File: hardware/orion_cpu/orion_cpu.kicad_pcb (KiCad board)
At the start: 2 copper layers, 99.7 x 99.7 mm, 74 parts, among them J1 C96ABC, J2 JTAG, SW1 CONFIG, SW2 ROM1, SW3 RESET

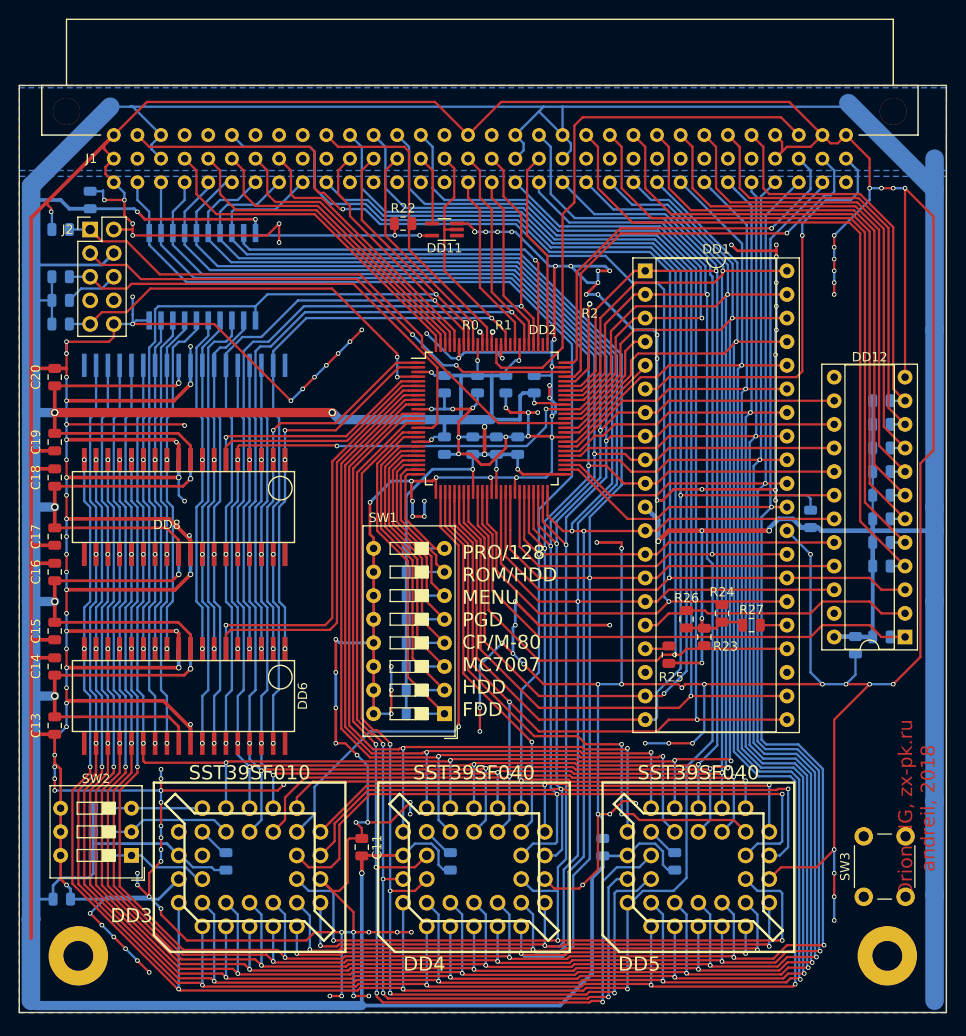
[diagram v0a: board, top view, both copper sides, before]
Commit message: RC версия процессорного модуля
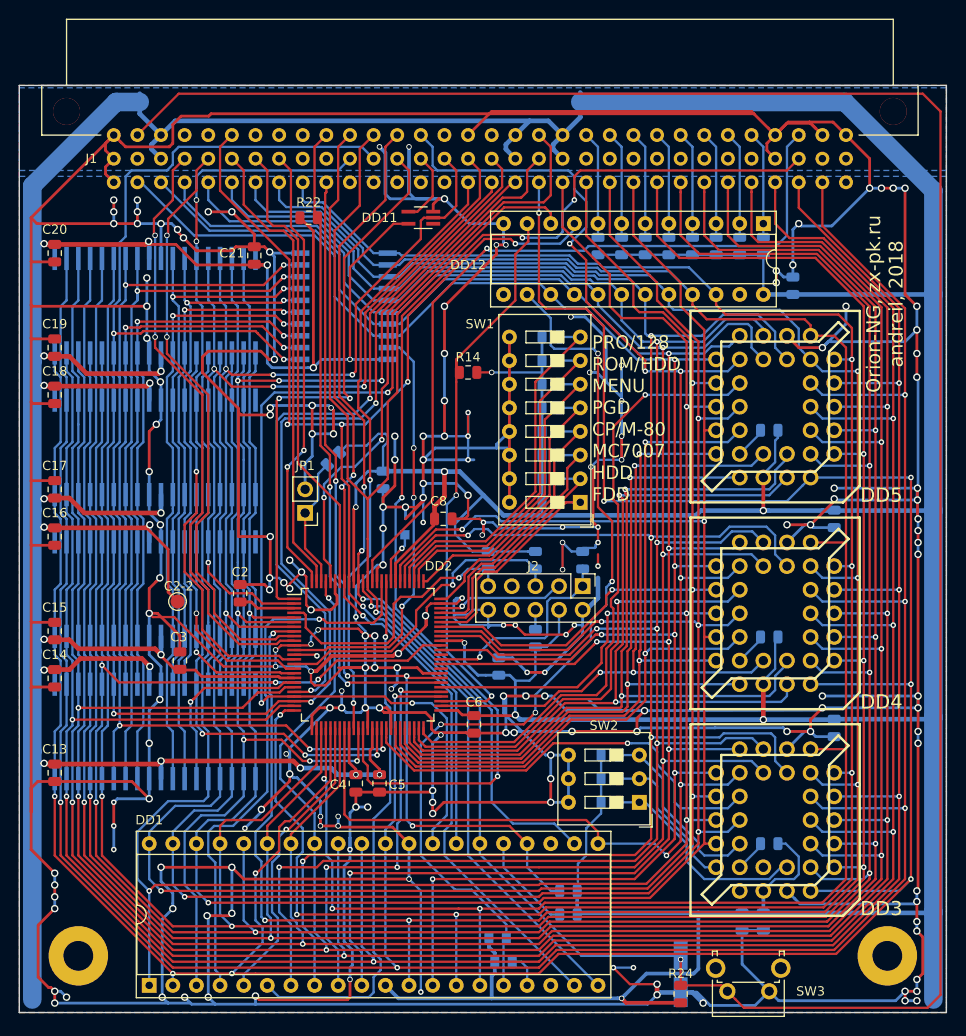
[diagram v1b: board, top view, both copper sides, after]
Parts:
- added C2-2: TestPoint_Pad_D1.5mm, TestPoint:TestPoint_Pad_D1.5mm, F.Cu at (86.9, 95.2)
- added C23: CP, Capacitors_Tantalum_SMD:CP_Tantalum_Case-A_EIA-3216-18_Hand, B.Cu at (141.0, 135.3)
- added JP1: R16B, Pin_Headers:Pin_Header_Straight_1x02_Pitch2.54mm, F.Cu at (100.6, 85.7)
- added R34: 1K, Resistor_SMD:R_0805_2012Metric, B.Cu at (103.6, 79.9)
- added REF**: TestPoint_Pad_1.0x1.0mm, TestPoint:TestPoint_Pad_1.0x1.0mm, B.Cu at (111.3, 88.1)
- C11, DD6, DD8, R23, R25, R26, R27: moved to B.Cu
- C2, C21, C3, C4, C5, C6, C8, R14: moved to F.Cu
- SW3: footprint Buttons_Switches_ThroughHole:SW_PUSH_6mm -> Button_Switch_THT:SW_Tactile_SPST_Angled_PTS645Vx83-2LFS
- moved DD1 93.5 mm to (83.8, 136.5), turned to 90 degrees
- moved C10 75.5 mm to (149.9, 129.7), turned to 90 degrees
- moved R32 66.4 mm to (130.4, 90.8), turned to 270 degrees
- moved J2 65.4 mm to (130.4, 93.6), turned to 270 degrees
- moved R29 62.7 mm to (125.3, 99.2), turned to 90 degrees
- moved R30 59.5 mm to (125.3, 90.8), turned to 270 degrees
- moved R12 58.5 mm to (150.5, 121.3), turned to 180 degrees
- moved DD3 56.7 mm to (151.1, 118.7), turned to 0 degrees
- moved R10 54.9 mm to (133.3, 114.3)
- moved R11 54.9 mm to (133.3, 111.8)
- moved R9 54.9 mm to (133.3, 116.8)
- moved SW2 54.9 mm to (136.5, 116.8)
- moved R14 52.8 mm to (118.1, 70.6), turned to 180 degrees
- moved R31 52.5 mm to (120.3, 90.8), turned to 270 degrees
- moved C11 52.4 mm to (157.5, 108.8), turned to 90 degrees
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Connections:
- net Net-(DD3-Pad31) renamed /PGM1
- net Net-(DD4-Pad31) renamed /PGM2
- net Net-(DD5-Pad31) renamed /PGM3
- DD10 pad 11: /D7 -> /D0
- DD10 pad 12: /D6 -> /D1
- DD10 pad 13: /D5 -> /D2
- DD10 pad 14: /D4 -> /D3
- DD10 pad 15: /D3 -> /D4
- DD10 pad 16: /D2 -> /D5
- DD10 pad 17: /D1 -> /D6
- DD10 pad 18: /D0 -> /D7
- DD10 pad 2: /MD7 -> /MD3
- DD10 pad 3: /MD0 -> /MD2
- DD10 pad 4: /MD6 -> /MD1
- DD10 pad 5: /MD1 -> /MD0
- DD10 pad 6: /MD2 -> /MD7
- DD10 pad 7: /MD5 -> /MD6
- DD10 pad 8: /MD3 -> /MD5
- DD12 pad 1: /~IRQ0 -> /~IRQS
- DD12 pad 10: /~IRQ7 -> /~IORQ
- DD12 pad 11: /~IRQS -> /~IRQ0
- DD12 pad 14: /D4 -> /~INT
- DD12 pad 15: /D3 -> /D7
- DD12 pad 16: /D5 -> /D6
- DD12 pad 17: /D6 -> /D5
- DD12 pad 18: /~IORQ -> /D4
- DD12 pad 19: /D2 -> /D3
- DD12 pad 2: /~INT -> /~IRQ7
- DD12 pad 20: /D7 -> /D2
- DD12 pad 21: /D0 -> /D1
- DD12 pad 22: /D1 -> /D0
- DD12 pad 3: /~M1 -> /~IRQ6
- DD12 pad 4: /~IRQ1 -> /~IRQ5
- DD12 pad 5: /~IRQ2 -> /~IRQ4
- DD12 pad 7: /~IRQ4 -> /~IRQ2
- DD12 pad 8: /~IRQ5 -> /~IRQ1
- DD12 pad 9: /~IRQ6 -> /~M1
- DD2 pad 1: /MA17 -> /~VCE
- DD2 pad 10: /R2A14 -> /~VO0
- DD2 pad 100: /~VO0 -> /pFA
- DD2 pad 12: /R2A17 -> /~OE0
- DD2 pad 13: /R2A18 -> /~OE1
- DD2 pad 14: /R2A16 -> /~CE0
- DD2 pad 16: /R2A15 -> /~CE1
- DD2 pad 17: /CFG0 -> /~CE2
- DD2 pad 19: /CFG1 -> /~CE3
- DD2 pad 2: /MA18 -> /MA15
- DD2 pad 20: /CFG2 -> /A2
- DD2 pad 21: /CFG3 -> /A14
- DD2 pad 22: /CFG4 -> /~RFSH
- DD2 pad 23: /CFG5 -> /MA14
- DD2 pad 24: /CFG6 -> /A1
- DD2 pad 25: /CFG7 -> /D0
- DD2 pad 27: /~R1 -> /A7
- DD2 pad 28: /~R2 -> /A5
- DD2 pad 29: /~R3 -> /D1
- DD2 pad 30: /~RD -> /A12
- DD2 pad 31: /~IORQ -> /ZA15
- DD2 pad 32: /~WR -> /A4
- DD2 pad 33: /~MREQ -> /~RD
- DD2 pad 35: /~WAIT -> /A15
- DD2 pad 36: /~IRQ0 -> /A13
- DD2 pad 37: /~RES -> /INT50
- DD2 pad 40: /D1 -> /~MRD
- DD2 pad 41: /~M1 -> /~MWR
- DD2 pad 42: /D0 -> /~R1
- DD2 pad 44: /~RFSH -> /R2A13
- DD2 pad 45: /D7 -> /R2A14
- DD2 pad 46: /D6 -> /R2A17
- DD2 pad 47: /D5 -> /R2A15
- DD2 pad 48: /D4 -> /R2A16
- DD2 pad 49: /D3 -> /~R2
- DD2 pad 5: /~CE3 -> /MA18
- DD2 pad 50: /D2 -> /~R3
- DD2 pad 52: /A0 -> /R2A18
- DD2 pad 53: /A1 -> /~IRQ0
- DD2 pad 54: /A2 -> /A0
- DD2 pad 55: /A3 -> /D5
- DD2 pad 56: /A4 -> /A11
- DD2 pad 57: /A5 -> /~BLIO
- DD2 pad 58: /A6 -> /~WAIT
- DD2 pad 6: /~CE2 -> /MA17
- DD2 pad 60: /ZA15 -> /CSL
- DD2 pad 61: /A7 -> /D6
- DD2 pad 63: /ZA14 -> /pFB
- DD2 pad 64: /A8 -> /D7
- DD2 pad 65: /A13 -> /A6
- DD2 pad 67: /A9 -> /D4
- DD2 pad 68: /A12 -> /A9
- DD2 pad 7: /~CE1 -> /MA16
- DD2 pad 70: /A11 -> /CFG0
- DD2 pad 71: /r2 -> /CFG1
- DD2 pad 72: /~TRB -> /CFG2
- DD2 pad 75: /INT50 -> /CFG3
- DD2 pad 76: /SND -> /CFG4
- DD2 pad 77: Net-(DD2-Pad77) -> /CFG5
- DD2 pad 78: /~OE0 -> /CFG6
- DD2 pad 79: /MA14 -> /CFG7
- DD2 pad 8: /~CE0 -> /D2
- DD2 pad 80: /A14 -> /D3
- DD2 pad 81: /MA15 -> /A8
- DD2 pad 83: /A15 -> Net-(DD2-Pad83)
- DD2 pad 84: Net-(DD2-Pad84) -> /ZCLK
- DD2 pad 85: /MA16 -> /ZA14
- DD2 pad 88: /R1 -> /~IORQ
- DD2 pad 89: /~BLIO -> /~RES
- DD2 pad 9: /R2A13 -> /~VO1
- DD2 pad 90: /R0 -> /~WR
- DD2 pad 92: /~VCE -> /~M1
- DD2 pad 93: /~MWR -> /~MREQ
- DD2 pad 94: /~MRD -> /pF8
- DD2 pad 96: /pFA -> /SND
- DD2 pad 97: /pF8 -> /A3
- DD2 pad 98: /pFC -> /R16B
- DD2 pad 99: /~VO1 -> /pFC
- DD3 pad 22: /~R1 -> /~RD
- DD3 pad 24: /~RD -> /~R1
- DD4 pad 22: /~R2 -> /~RD
- DD4 pad 24: /~RD -> /~R2
- DD5 pad 22: /~R3 -> /~RD
- DD5 pad 24: /~RD -> /~R3
- DD6 pad 1: /MA18 -> /A8
- DD6 pad 14: /A0 -> /A7
- DD6 pad 15: /A2 -> /A5
- DD6 pad 16: /A4 -> /A3
- DD6 pad 17: /A6 -> /A1
- DD6 pad 2: /MA17 -> /A13
- DD6 pad 20: /A7 -> /A0
- DD6 pad 21: /A5 -> /A2
- DD6 pad 22: /A3 -> /A4
- DD6 pad 23: /A1 -> /A6
- DD6 pad 24: /A8 -> /MA14
- DD6 pad 3: /MA15 -> /A9
- DD6 pad 32: /A11 -> /MA15
- DD6 pad 33: /A9 -> /MA16
- DD6 pad 34: /A10 -> /MA17
- DD6 pad 35: /MA16 -> /MA18
- DD6 pad 4: /MA14 -> /A10
- DD6 pad 5: /A13 -> /A11
- DD7 pad 1: /MA18 -> /A8
- DD7 pad 14: /A0 -> /A7
- DD7 pad 15: /A2 -> /A5
- DD7 pad 16: /A4 -> /A3
- DD7 pad 17: /A6 -> /A1
- DD7 pad 2: /MA17 -> /A13
- DD7 pad 20: /A7 -> /A0
- DD7 pad 21: /A5 -> /A2
- DD7 pad 22: /A3 -> /A4
- DD7 pad 23: /A1 -> /A6
- DD7 pad 24: /A8 -> /MA14
- DD7 pad 3: /MA15 -> /A9
- DD7 pad 32: /A11 -> /MA15
- DD7 pad 33: /A9 -> /MA16
- DD7 pad 34: /A10 -> /MA17
- DD7 pad 35: /MA16 -> /MA18
- DD7 pad 4: /MA14 -> /A10
- DD7 pad 5: /A13 -> /A11
- DD8 pad 1: /MA18 -> /A8
- DD8 pad 14: /A0 -> /A7
- DD8 pad 15: /A2 -> /A5
- DD8 pad 16: /A4 -> /A3
- DD8 pad 17: /A6 -> /A1
- DD8 pad 2: /MA17 -> /A13
- DD8 pad 20: /A7 -> /A0
- DD8 pad 21: /A5 -> /A2
- DD8 pad 22: /A3 -> /A4
- DD8 pad 23: /A1 -> /A6
- DD8 pad 24: /A8 -> /MA14
- DD8 pad 3: /MA15 -> /A9
- DD8 pad 32: /A11 -> /MA15
- DD8 pad 33: /A9 -> /MA16
- DD8 pad 34: /A10 -> /MA17
- DD8 pad 35: /MA16 -> /MA18
- DD8 pad 4: /MA14 -> /A10
- DD8 pad 5: /A13 -> /A11
- DD9 pad 1: /MA18 -> /A8
- DD9 pad 14: /A0 -> /A7
- DD9 pad 15: /A2 -> /A5
- DD9 pad 16: /A4 -> /A3
- DD9 pad 17: /A6 -> /A1
- DD9 pad 2: /MA17 -> /A13
- DD9 pad 20: /A7 -> /A0
- DD9 pad 21: /A5 -> /A2
- DD9 pad 22: /A3 -> /A4
- DD9 pad 23: /A1 -> /A6
- DD9 pad 24: /A8 -> /MA14
- DD9 pad 3: /MA15 -> /A9
- DD9 pad 32: /A11 -> /MA15
- DD9 pad 33: /A9 -> /MA16
- DD9 pad 34: /A10 -> /MA17
- DD9 pad 35: /MA16 -> /MA18
- DD9 pad 4: /MA14 -> /A10
- DD9 pad 5: /A13 -> /A11
- J1 pad 31b: /~TRB -> Net-(J1-Pad31b)
- J1 pad 32b: /ZCLK -> Net-(J1-Pad32b)
- R10 pad 2: /R1A13 -> /R1A14
- R11 pad 2: /R1A14 -> /R1A13
- SW2 pad 2: /R1A13 -> /R1A14
- SW2 pad 3: /R1A14 -> /R1A13
- SW3 pad 1: Net-(SW3-Pad1) -> GND
- SW3 pad 2: Net-(SW3-Pad2) -> /~RES
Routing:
- net GND: track 1226.9 -> 1522.7 mm, vias 186 -> 198
- net /~RES: track 143.0 -> 277.8 mm
- net /INT50: track 43.4 -> 127.2 mm, vias 1 -> 4
- net /A12: track 259.8 -> 329.3 mm, vias 7 -> 9
- net /~INT: track 29.8 -> 99.2 mm, vias 0 -> 4
- net /~IRQ1: track 75.8 -> 11.5 mm
- net /MA14: track 86.5 -> 148.8 mm
- net /~IRQ2: track 71.1 -> 11.5 mm
- net VCC: track 912.1 -> 969.0 mm, vias 29 -> 30
- net /~IRQ3: track 66.4 -> 11.5 mm
- net /A14: track 19.2 -> 73.6 mm, vias 0 -> 2
- net /~MWR: track 95.3 -> 149.3 mm, vias 3 -> 5
- net /~IRQ4: track 61.7 -> 11.5 mm
- net /A11: track 207.2 -> 256.6 mm, vias 6 -> 5
- net /~RD: track 218.0 -> 168.7 mm, vias 4 -> 6
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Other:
- net class Default: clearance 0.175 -> 0.176
- rule trace_clearance: 0.175 -> 0.176
- rule trace_min: 0.16 -> 0.17
- board text removed: "R0"
- board text removed: "R1"
- board text removed: "R2"
